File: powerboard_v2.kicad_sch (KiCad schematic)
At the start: 17 parts, among them J1 Conn_01x02_Pin, J4 Conn_01x02_Pin, J5 Conn_01x02_Pin, K3 Relay_SPDT, K4 Relay_SPDT, U5 TLP785

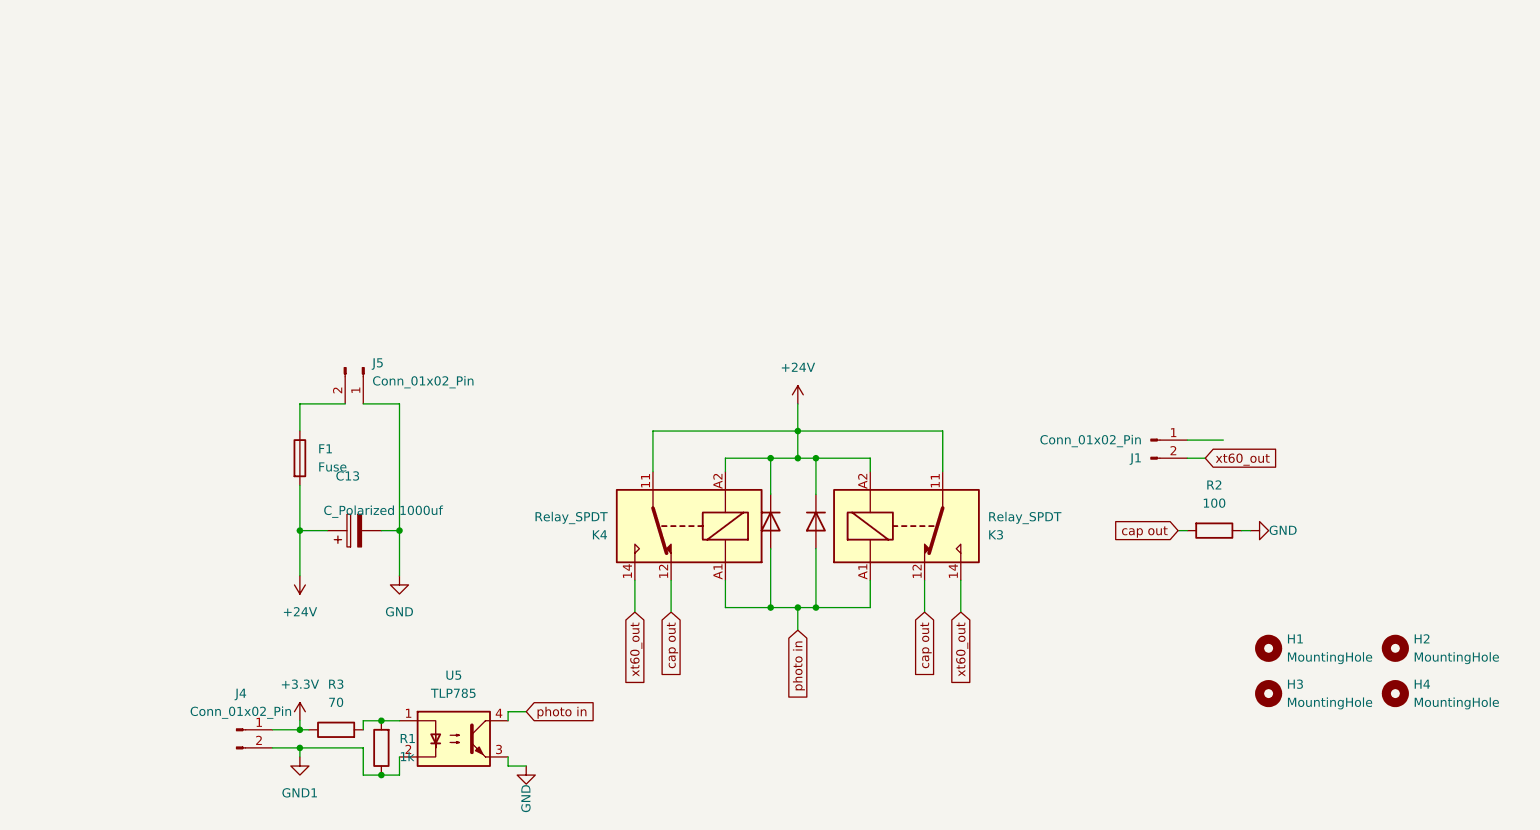
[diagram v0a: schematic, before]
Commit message: 配線前最終版
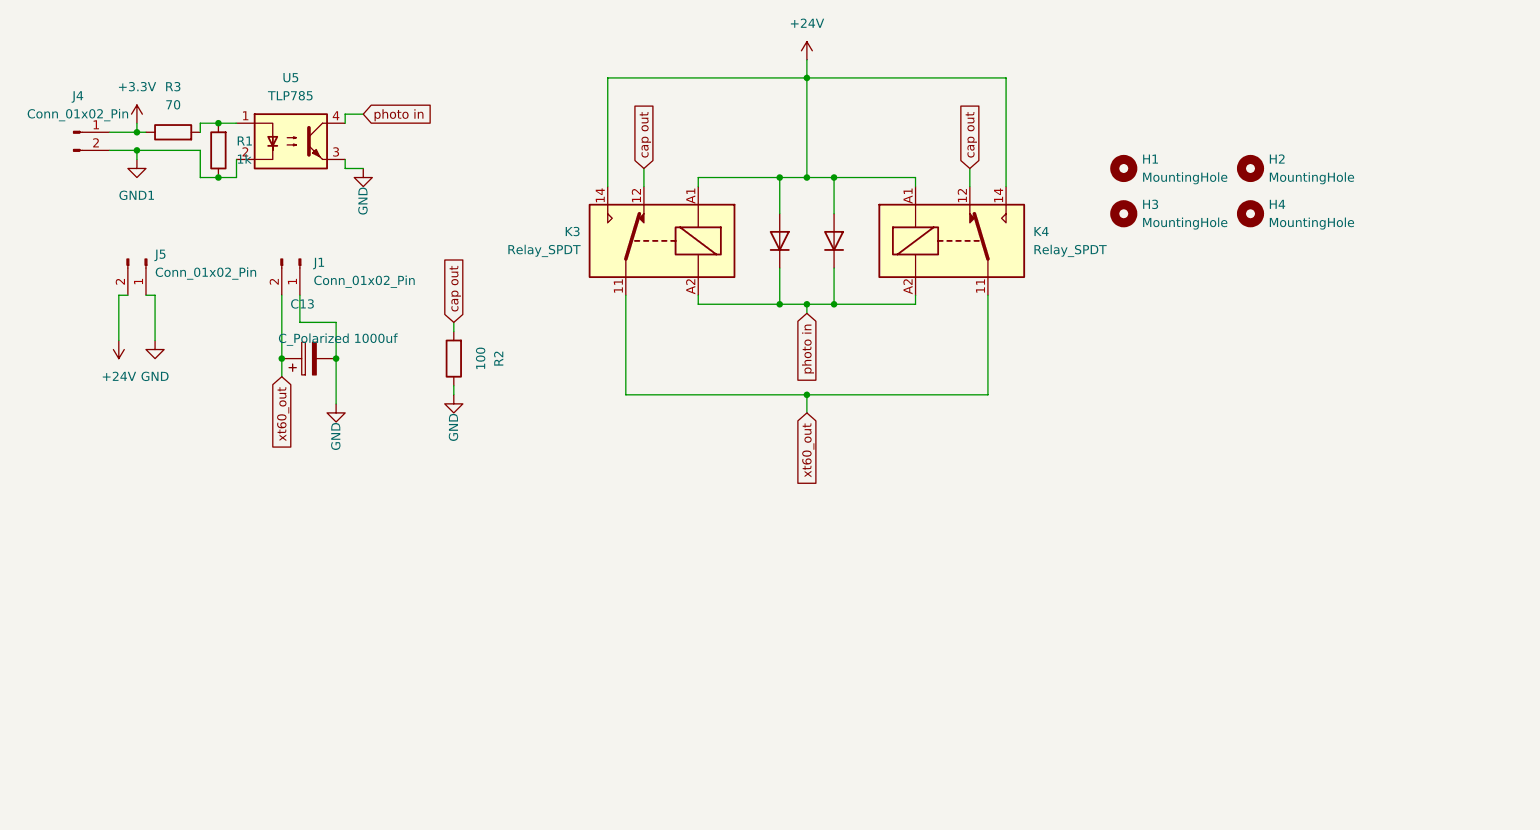
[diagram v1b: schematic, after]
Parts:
- removed F1: Fuse, Fuse:Fuseholder_Blade_ATO_Littelfuse_Pudenz_2_Pin, symbol Device:Fuse
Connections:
- net +24V: now also D1.2 (A), D3.2 (A), J5.2 (Pin_2), K3.14, K3.A1, K4.14, K4.A1; no longer C13.1, D1.1 (K), D3.1 (K), K3.11, K3.A2, K4.11, K4.A2
- net GND: now also J1.1 (Pin_1)
- net photo in: now also D1.1 (K), D3.1 (K), K3.A2, K4.A2; no longer D1.2 (A), D3.2 (A), K3.A1, K4.A1
- net xt60_out: now also C13.1, K3.11, K4.11; no longer K3.14, K4.14
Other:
- moved on the sheet: C13, H1, H2, H3, H4, J1, J4, J5, K3, K4, R1, R2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
